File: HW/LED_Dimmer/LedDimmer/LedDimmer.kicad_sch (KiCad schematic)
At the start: 60 parts, among them J1 Screw_Terminal_01x03, J2 Screw_Terminal_01x02, J3 Screw_Terminal_01x03, J4 Screw_Terminal_01x03, J5 Screw_Terminal_01x03, J6 Screw_Terminal_01x02, Q1 SSM3J133TU, Q2 BSS138, Q3 BSS138, Q4 SSM3J133TU, U1 TPS561243, U2 PIC12F1572, U3 TPS629203-Q1

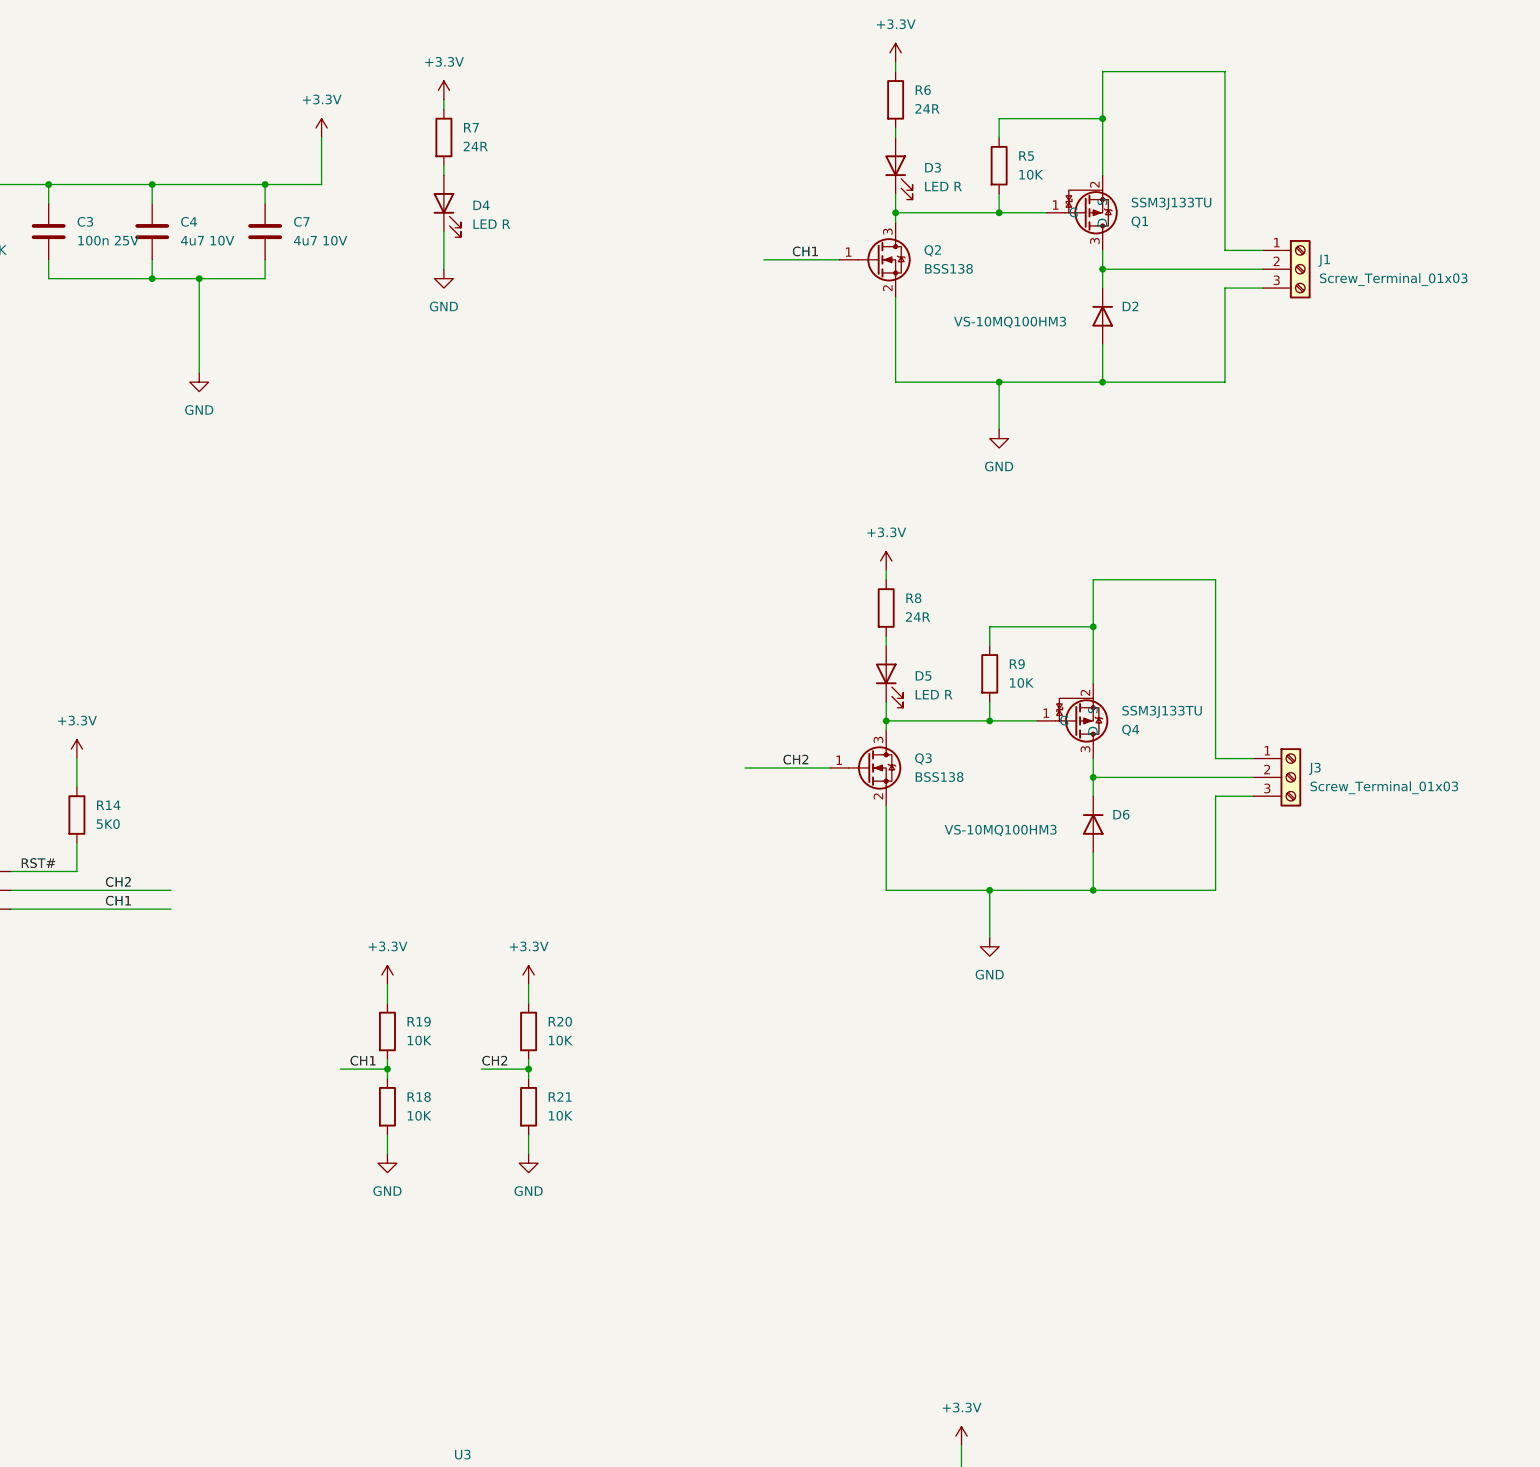
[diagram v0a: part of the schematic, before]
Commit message: .
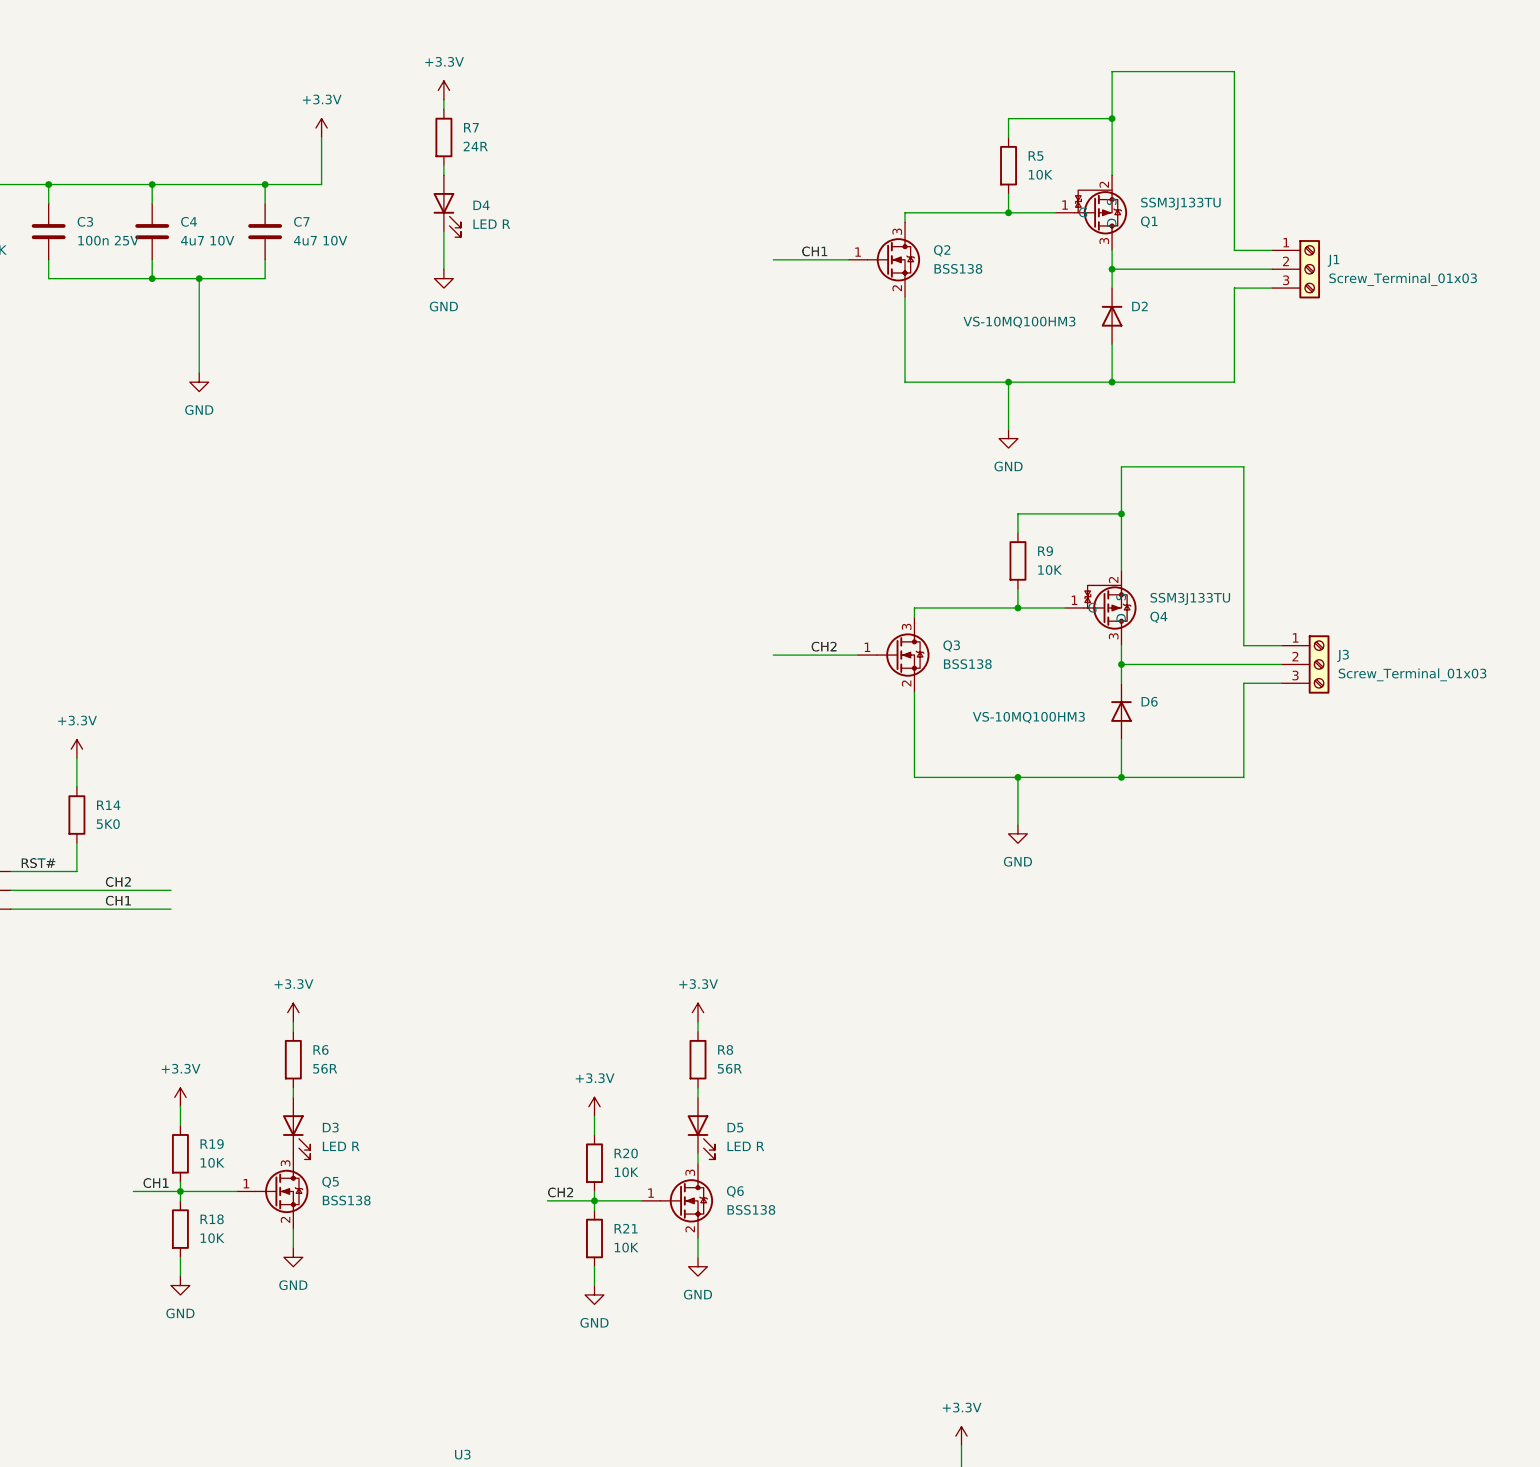
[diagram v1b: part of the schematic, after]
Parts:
- added Q5, Q6: BSS138, Package_TO_SOT_SMD:SOT-23, symbol bt_transistor:T;Mn;BSS138;SOT23
- R6, R8: value 24R -> 56R; symbol bt_resistors:R;G;24R;10P0;S;0603 -> bt_resistors:R;G;56R;10P0;S;0603; CPN BT00002-00240 -> BT00002-00560
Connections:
- net CH1: now also Q5.1 (G)
- net CH2: now also Q6.1 (G)
- net GND: now also Q5.2 (S), Q6.2 (S)
- net at Q3.3 (D), Q4.1 (G), R9.2: no longer D5.1 (K)
- net at Q1.1 (G), Q2.3 (D), R5.2: no longer D3.1 (K)
- new net: D3.1 (K), Q5.3 (D)
- new net: D5.1 (K), Q6.3 (D)
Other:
- moved on the sheet: D2, D3, D5, D6, J1, J3, Q1, Q2, Q3, Q4, R18, R19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
